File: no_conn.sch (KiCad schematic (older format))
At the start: 0 parts

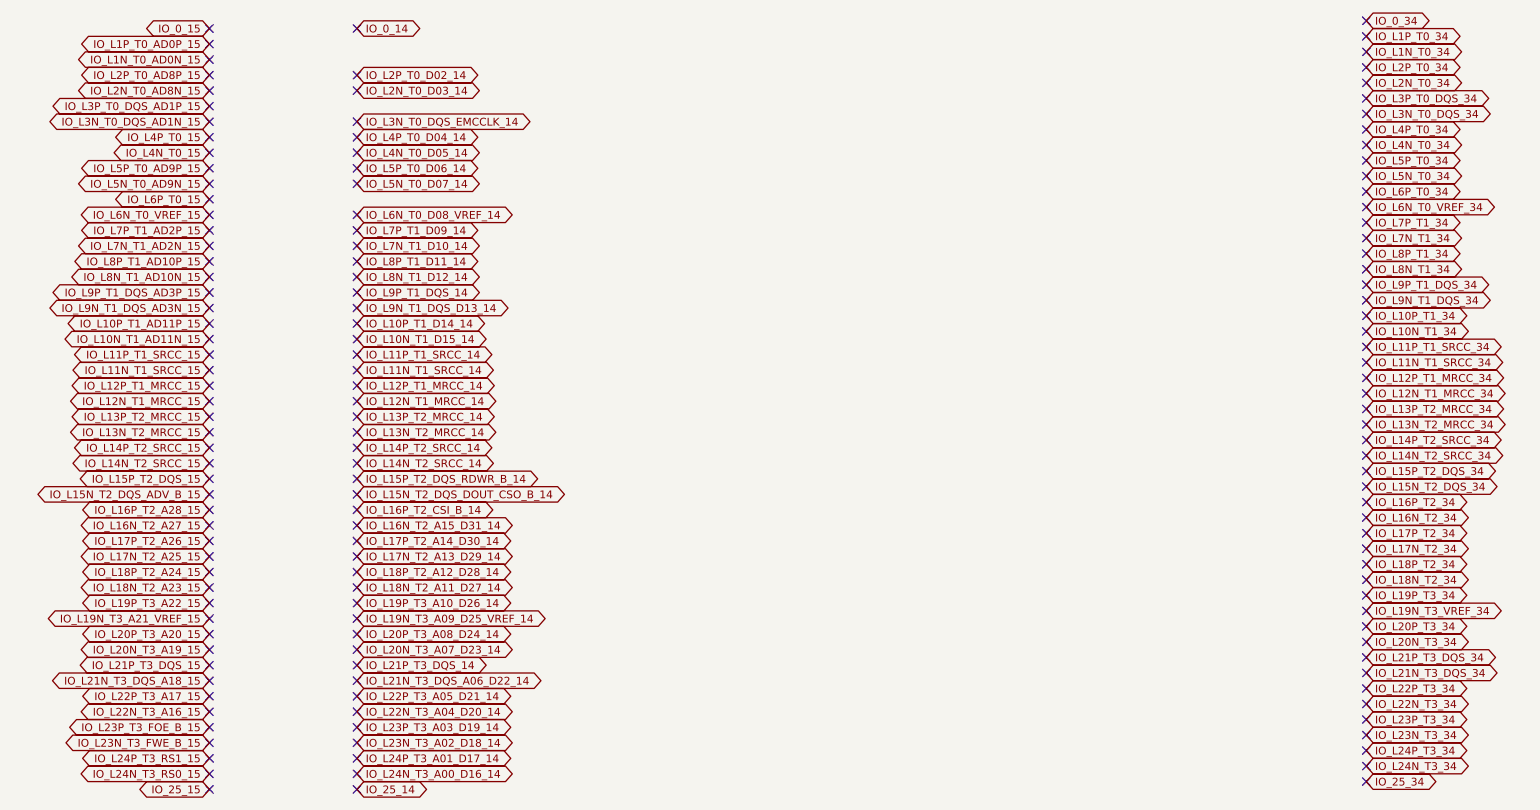
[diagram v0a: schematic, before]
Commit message: WIP: point before we change to OSH/relaxed process
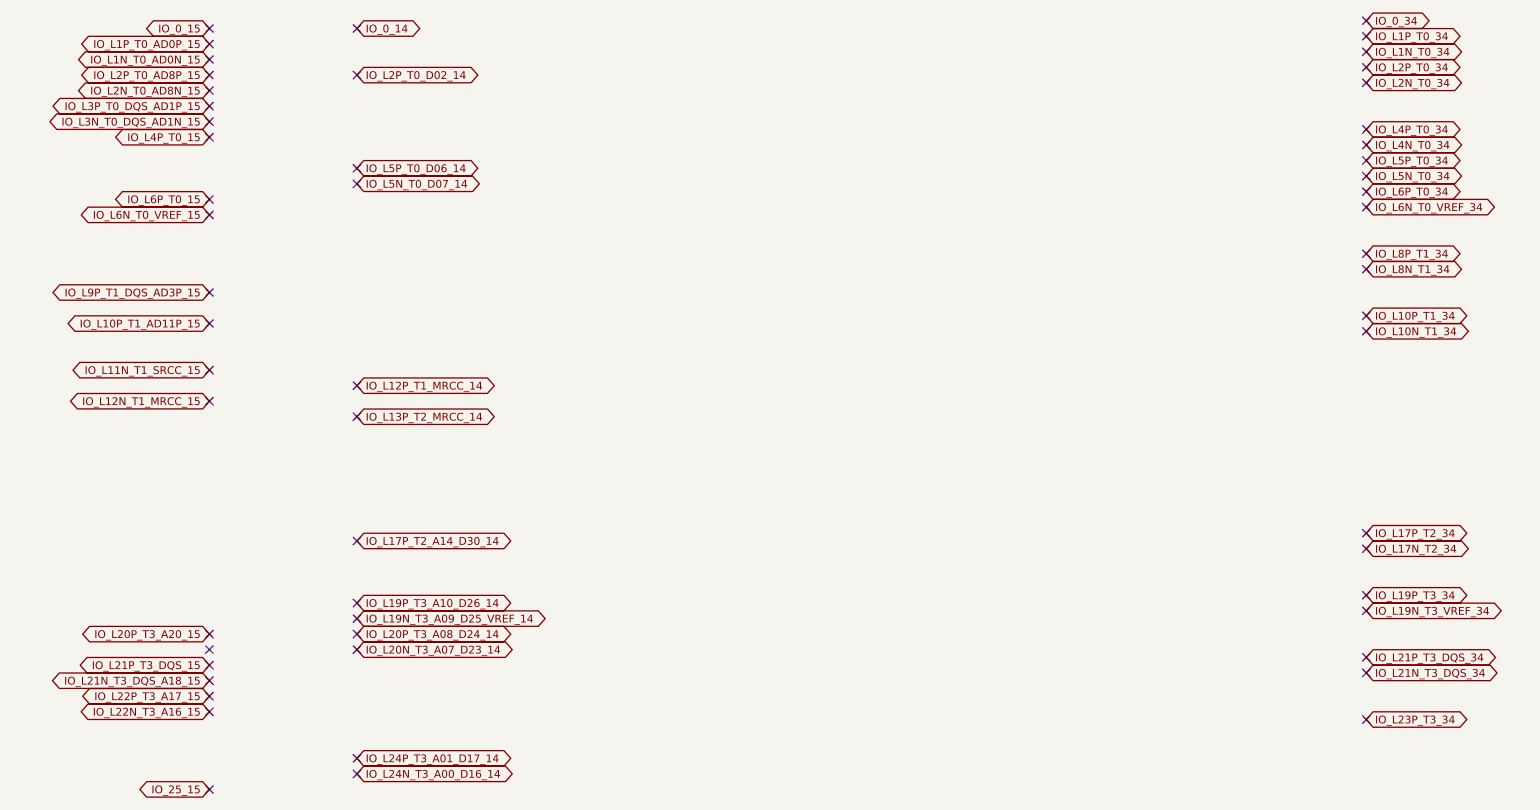
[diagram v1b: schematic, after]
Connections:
- no-connect marks 146 -> 56
